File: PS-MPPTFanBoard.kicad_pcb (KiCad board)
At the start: 2 copper layers, 100 x 49 mm, 137 parts, among them IC1 TCAN3413DR, IC2 LM74502DDFR, IC3 TCAN3413DR, J11 USB_C_Receptacle_USB2.0_16P, J5 SWD_Header, J6 SWD, Q1 PSMN012-100YS, Q2 PSMN012-100YS, SW1 Reset, SW2 SW_SPDT, U1 EMC2305-1-AP-TR, U2 STM32G473CETx, U3 MCP1826S, U4 LMR51635XDDCR, U5 TPS2117DRLR, Y1 Crystal

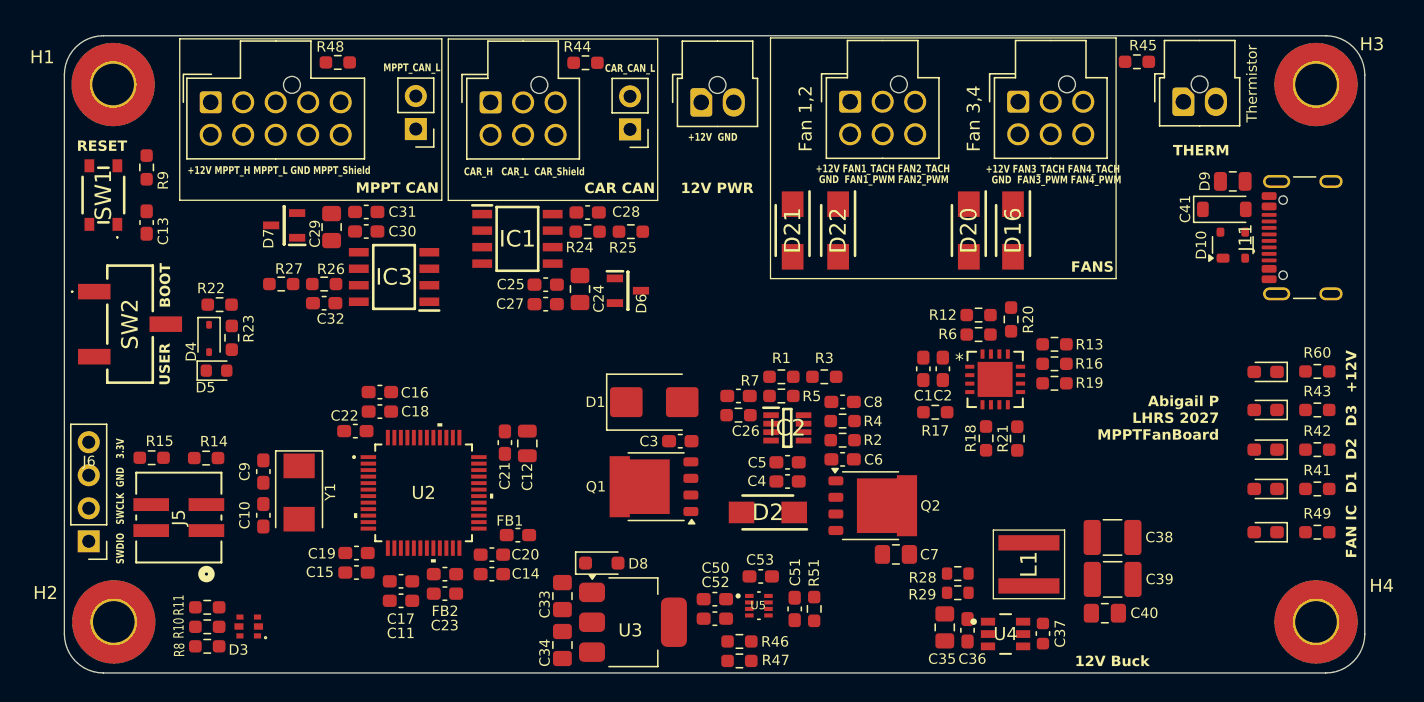
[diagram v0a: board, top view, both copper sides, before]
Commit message: routing
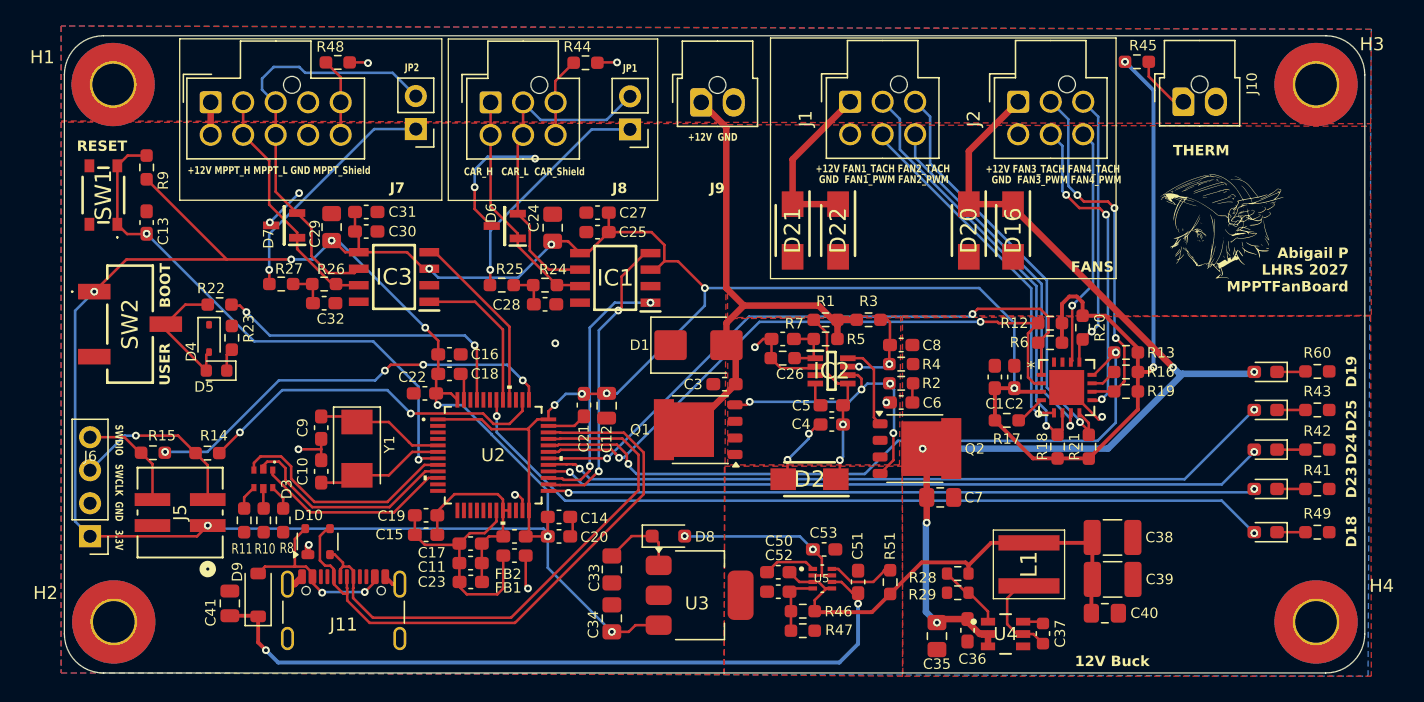
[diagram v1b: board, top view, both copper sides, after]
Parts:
- added G***: LOGO, LOGO, F.Cu at (167.5, 67.8)
- D18: renamed from FAN IC
- J1: renamed from Fan 1,2
- J2: renamed from Fan 3,4
- J7: renamed from MPPT CAN
- J8: renamed from CAR CAN
- J9: renamed from 12V PWR
- moved C41 83.7 mm to (91.2, 96.9), turned to -90 degrees
- moved J11 80.5 mm to (100.0, 98.5), turned to 0 degrees
- moved D9 80.0 mm to (93.4, 96.2), turned to 90 degrees
- moved D10 74.0 mm to (98.0, 92.2)
- moved LOGO4 15.2 mm to (170.5, 74.8)
- moved D3 11.4 mm to (93.8, 87.3), turned to -90 degrees
- moved R8 11.3 mm to (95.3, 90.5), turned to -90 degrees
- moved R25 10.7 mm to (112.1, 72.4), turned to 180 degrees
- moved D6 10.7 mm to (112.4, 67.9), turned to 180 degrees
- moved R10 9.27 mm to (93.8, 90.5), turned to -90 degrees
- moved IC1 8.10 mm to (120.9, 71.9), turned to 180 degrees
- moved C27 8.09 mm to (119.5, 66.8), turned to 180 degrees
- moved C28 7.78 mm to (115.5, 73.9), turned to 180 degrees
- moved R11 7.26 mm to (92.3, 90.5), turned to -90 degrees
- moved C14 6.78 mm to (116.5, 90.2), turned to 0 degrees
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- renumbered +12V to D19, D1 to D23, D2 to D24, D3 to D25, Thermistor to J10, CAR_CAN_L to JP1, MPPT_CAN_L to JP2
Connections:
- U2 pad 11: /DEBUG1 -> /48PinMCU/PA3
- U2 pad 12: /DEBUG2 -> /48PinMCU/PA4
- U2 pad 13: /DEBUG3 -> /48PinMCU/PA5
- U2 pad 25: /48PinMCU/PB11 -> /DEBUG1
- U2 pad 28: /48PinMCU/PB14 -> /DEBUG2
- U2 pad 29: /48PinMCU/PB15 -> /DEBUG3
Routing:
- net +3.3V: track 0.00 -> 301.0 mm, vias 0 -> 17
- net +12V: track 0.00 -> 94.6 mm, vias 0 -> 5
- net /FAN_CHIP: track 0.00 -> 64.0 mm, vias 0 -> 2
- net /USB_5V: track 0.00 -> 57.8 mm, vias 0 -> 2
- net /DEBUG3: track 0.00 -> 57.0 mm, vias 0 -> 2
- net /DEBUG2: track 0.00 -> 55.9 mm, vias 0 -> 2
- net /~{SMBALERT}: track 0.00 -> 54.7 mm, vias 0 -> 2
- net GND: track 0.00 -> 54.6 mm, vias 0 -> 16
- net /DEBUG1: track 0.00 -> 54.5 mm, vias 0 -> 2
- net /FAN_SDA: track 0.00 -> 48.4 mm, vias 0 -> 2
- net /FAN_SCL: track 0.00 -> 48.1 mm, vias 0 -> 2
- net /USB_D-: track 0.00 -> 47.3 mm
- net /48PinMCU/NRST: track 0.00 -> 42.6 mm, vias 0 -> 2
- net /USB_D+: track 0.00 -> 42.3 mm
- net /12V_In: track 0.00 -> 39.6 mm
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- added copper zone on F.Cu, net +12V
- added copper zone on F.Cu, net /PowerProtection/source
- added copper zone on B.Cu, net GND
- added copper zone on F.Cu, net GND

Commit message: layout reviews
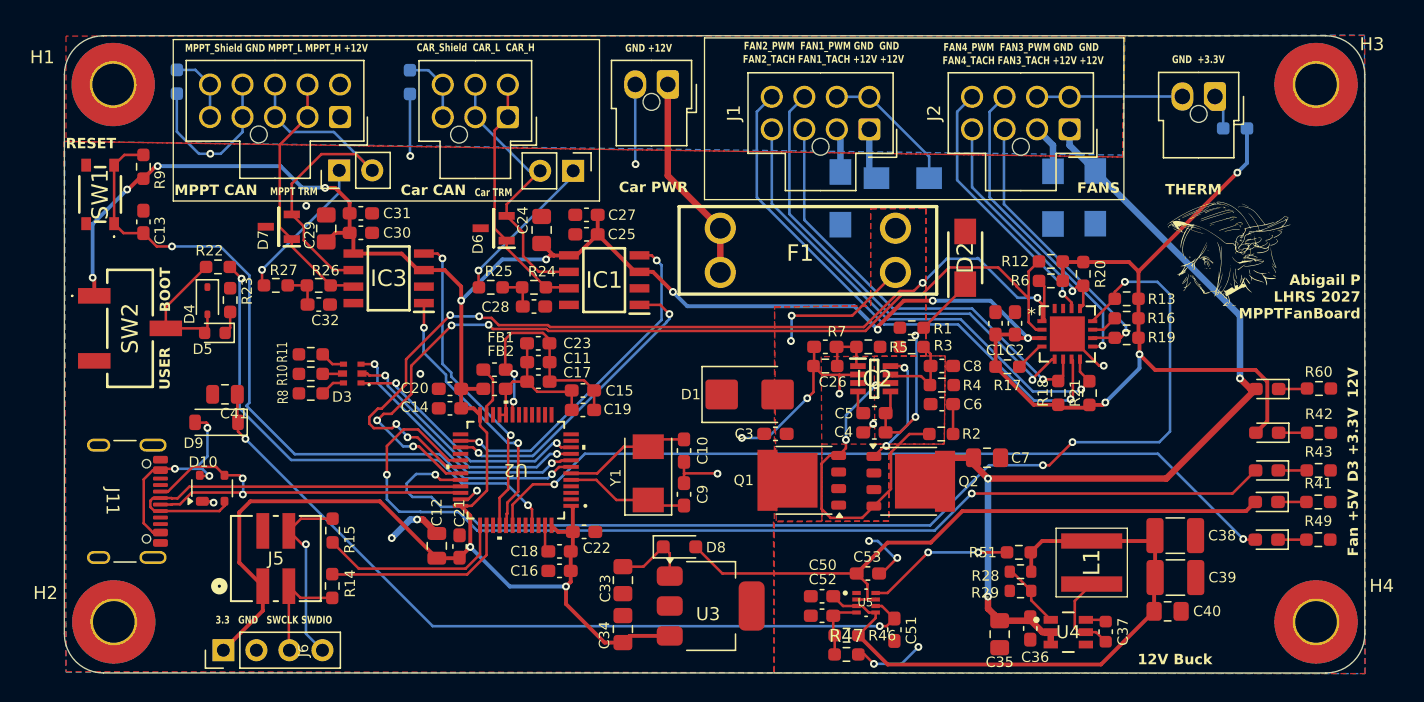
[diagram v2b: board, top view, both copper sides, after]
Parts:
- added F1: Fuse_3557_2, LHRS_Power:Fuse-3557-2, F.Cu at (135.7, 69.8)
- +3.3V: renamed from D24; value Debug2 -> 3.3V
- +5V: renamed from D23; value Debug1 -> 5V
- Car CAN: renamed from J8
- Car PWR: renamed from J9
- Car TRM: renamed from JP1
- D16, D20, D21, D22, R44, R45, R48: moved to B.Cu
- J1, J2: footprint LHRS_Connectors:Molex_Nano-Fit_105310-xx06_2x03_P2.50mm_Vertical -> LHRS_Connectors:Molex_Nano-Fit_105310-xx08_2x04_P2.50mm_Vertical
- MPPT CAN: renamed from J7
- MPPT TRM: renamed from JP2
- R47: value 3.6k -> 4.7k
- moved C9 28.4 mm to (126.2, 88.5), turned to -90 degrees
- moved C10 27.9 mm to (126.2, 85.2), turned to -90 degrees
- moved Y1 22.5 mm to (123.4, 86.9), turned to 90 degrees
- moved D2 20.8 mm to (147.8, 70.3), turned to 90 degrees
- moved J11 20.1 mm to (82.2, 89.0), turned to -90 degrees
- moved C23 19.1 mm to (114.9, 76.9), turned to 0 degrees
- moved C16 18.7 mm to (116.6, 94.4), turned to 180 degrees
- moved C12 16.9 mm to (107.1, 92.5), turned to 90 degrees
- moved C15 16.4 mm to (118.4, 80.5), turned to 0 degrees
- moved C11 16.3 mm to (115.0, 78.4), turned to 0 degrees
- moved C22 16.2 mm to (118.5, 91.4), turned to 0 degrees
- moved C41 16.1 mm to (90.8, 80.8), turned to 0 degrees
- moved C18 16.1 mm to (116.6, 92.9), turned to 180 degrees
- moved R15 15.1 mm to (99.1, 91.3), turned to 90 degrees
- moved C19 14.5 mm to (118.4, 82.0), turned to 0 degrees
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- renumbered D19 to 12V, D25 to D3, D18 to Fan, J10 to THERM
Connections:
- +3.3V pad 2: /DEBUG2 -> +3.3V
- +5V pad 2: /DEBUG1 -> +5V
- Car PWR pad 1: /12V_In -> Net-(J9-+12V)
- J1 pad 2: /FAN1_TACH -> +12V
- J1 pad 3: /FAN2_TACH -> /FAN1_TACH
- J1 pad 4: /FAN2_PWM -> /FAN2_TACH
- J1 pad 5: /FAN1_PWM -> /FAN2_PWM
- J1 pad 6: GND -> /FAN1_PWM
- J2 pad 2: /FAN3_TACH -> +12V
- J2 pad 3: /FAN4_TACH -> /FAN3_TACH
- J2 pad 4: /FAN4_PWM -> /FAN4_TACH
- J2 pad 5: /FAN3_PWM -> /FAN4_PWM
- J2 pad 6: GND -> /FAN3_PWM
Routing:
- net /DEBUG2: track 55.9 -> 0.00 mm, vias 2 -> 0
- net /DEBUG1: track 54.5 -> 0.00 mm, vias 2 -> 0
- net +3.3V: track 301.0 -> 247.3 mm, vias 17 -> 15
- net GND: track 54.6 -> 93.7 mm, vias 16 -> 19
- net +5V: track 14.0 -> 50.0 mm, vias 2 -> 0
- net /~{SMBALERT}: track 54.7 -> 86.5 mm, vias 2 -> 4
- net /12V_In: track 39.6 -> 11.3 mm, vias 0 -> 2
- net /FAN_SDA: track 48.4 -> 74.2 mm, vias 2 -> 6
- net /DEBUG3: track 57.0 -> 81.1 mm
- net /FAN_SCL: track 48.1 -> 72.0 mm, vias 2 -> 4
- net /48PinMCU/SWDIO: track 32.5 -> 14.8 mm, vias 4 -> 0
- net Net-(J9-+12V): track 0.00 -> 16.1 mm
- net /USB_D-: track 47.3 -> 32.2 mm, vias 0 -> 2
- net /48PinMCU/NRST: track 42.6 -> 56.9 mm
- net /48PinMCU/BOOT0: track 24.3 -> 38.3 mm
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- added copper zone on F.Cu, net /12V_In
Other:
- board text added: "3.3 GND SWCLK SWDIO"
- board text added: "CAR_Shield CAR_L CAR_H"
- board text added: "FAN2_PWM FAN1_PWM GND GND"
- board text added: "FAN2_TACH FAN1_TACH +12V +12V"
- board text added: "FAN4_PWM FAN3_PWM GND GND"
- board text added: "FAN4_TACH FAN3_TACH +12V +12V"
- board text added: "GND +12V"
- board text added: "GND +3.3V"
- board text added: "MPPT_Shield GND MPPT_L MPPT_H +12V"
- board text removed: "+12V FAN1_TACH FAN2_TACH"
- board text removed: "+12V FAN3_TACH FAN4_TACH"
- board text removed: "+12V GND"
- board text removed: "+12V MPPT_H MPPT_L GND MPPT_Shield"
- board text removed: "CAR_H CAR_L CAR_Shield"
- board text removed: "GND FAN1_PWM FAN2_PWM"
- board text removed: "GND FAN3_PWM FAN4_PWM"
- board text removed: "Note: I changed from 4 fan connectors to 2 2x3 for sizing purposes. Do I still need 4 diodes for the 4 fans or just 2 for the connectors. Should I have two ground and 12v pins on the fan connectors to acount for the two fans? If so, the can pin headers will not fit on the same row as the rest of the connectors"
- board text removed: "SWDIO SWCLK GND 3.3V"
- board text removed: "THERM"

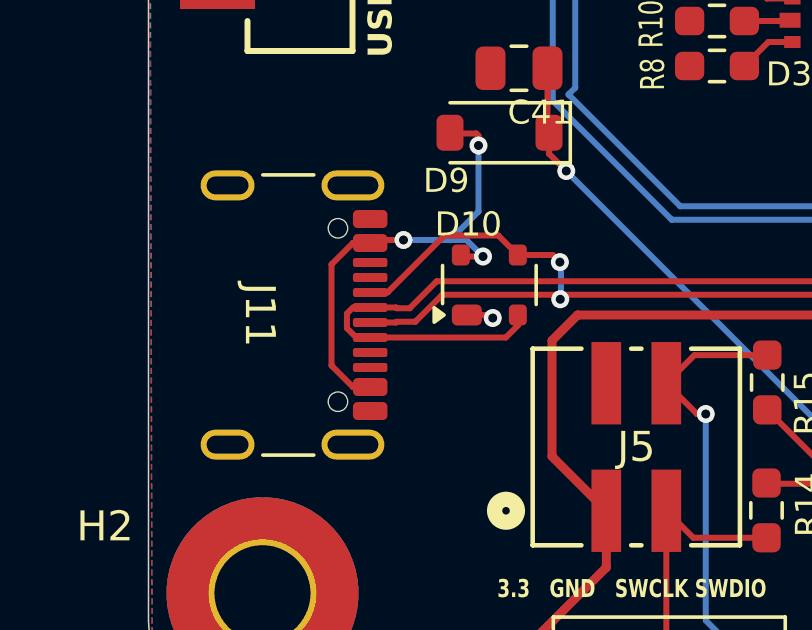
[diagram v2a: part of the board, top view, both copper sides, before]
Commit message: gnds
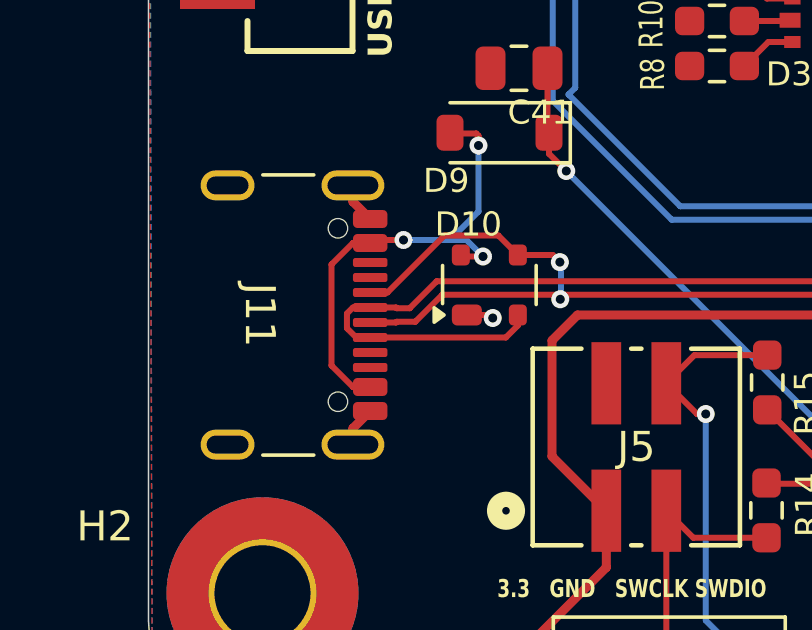
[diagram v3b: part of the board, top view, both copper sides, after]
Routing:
- net GND: track 93.7 -> 96.4 mm
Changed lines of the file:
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@@
+	)
+	(segment
+		(start 85.315 93.37)
+		(end 85.315 92.825)
+		(width 0.3)
+		(layer "F.Cu")
+		(net "GND")
 	)
 	(segment
@@
 		(end 110.225 88.225)
 		(width 0.2)
+		(layer "F.Cu")
+		(net "GND")
+	)
+	(segment
+		(start 85.315 84.73)
+		(end 85.315 85.275)
+		(width 0.3)
 		(layer "F.Cu")
 		(net "GND")
@@
 		(end 111.4514 79.6625)
 		(width 0.2)
+		(layer "F.Cu")
+		(net "GND")
+	)
+	(segment
+		(start 85.315 85.275)
+		(end 85.89 85.85)
+		(width 0.3)
 		(layer "F.Cu")
 		(net "GND")
@@
 		(layer "F.Cu")
 		(net "GND")
+	)
+	(segment
+		(start 85.315 92.825)
+		(end 85.89 92.25)
+		(width 0.3)
+		(layer "F.Cu")
+		(net "GND")
